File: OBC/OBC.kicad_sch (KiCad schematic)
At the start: 2 parts, among them J1 Conn_02x20_Odd_Even, U1 MPU9250

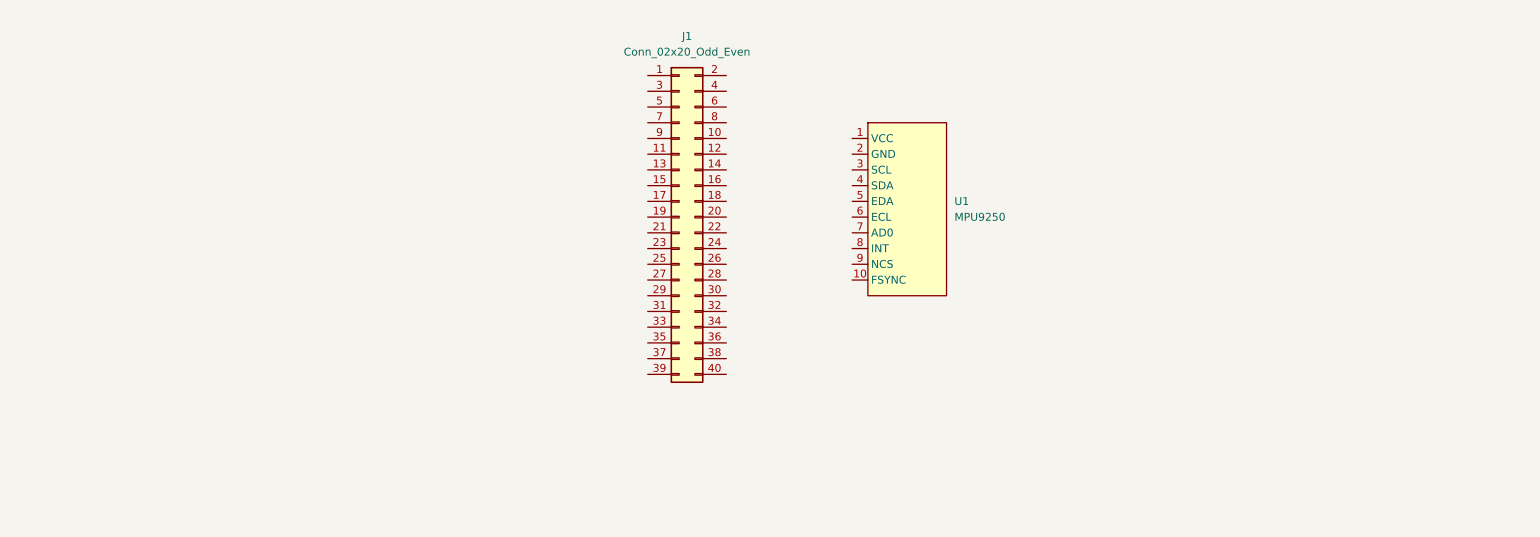
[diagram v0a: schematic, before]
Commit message: Agrega símbolo de rpi pi zero 2w
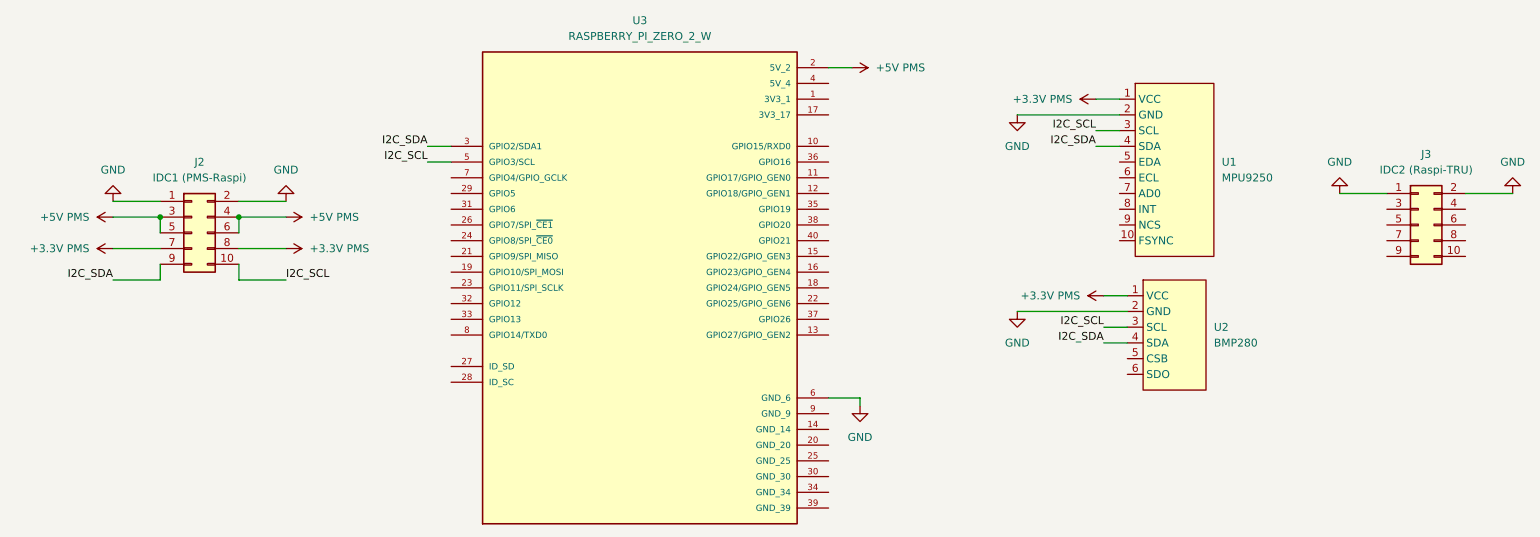
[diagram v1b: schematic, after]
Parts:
- removed J1: Conn_02x20_Odd_Even, symbol Connector_Generic:Conn_02x20_Odd_Even
- added J2: IDC1 (PMS-Raspi), symbol Connector_Generic:Conn_02x05_Odd_Even
- added J3: IDC2 (Raspi-TRU), symbol Connector_Generic:Conn_02x05_Odd_Even
- added U2: BMP280, symbol Cubesat:BMP280
- added U3: RASPBERRY_PI_ZERO_2_W, RASPBERRY_PI_ZERO_2_W:MODULE_RASPBERRY_PI_ZERO_2_W, symbol RASPBERRY_PI_ZERO_2_W:RASPBERRY_PI_ZERO_2_W
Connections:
- net +3.3V PMS: now reaches U1.1 (VCC)
- net +3.3V PMS: now also J2.7 (Pin_7), J2.8 (Pin_8), U2.1 (VCC)
- net GND: now reaches U1.2 (GND)
- net GND: now also J2.1 (Pin_1), J2.2 (Pin_2), J3.1 (Pin_1), J3.2 (Pin_2), U2.2 (GND), U3.6 (GND_6)
- net I2C_SCL: now reaches U1.3 (SCL)
- net I2C_SCL: now also J2.10 (Pin_10), U2.3 (SCL), U3.5 (GPIO3/SCL)
- net I2C_SDA: now reaches U1.4 (SDA)
- net I2C_SDA: now also J2.9 (Pin_9), U2.4 (SDA), U3.3 (GPIO2/SDA1)
- new net +5V PMS: J2.3 (Pin_3), J2.4 (Pin_4), J2.5 (Pin_5), J2.6 (Pin_6), U3.2 (5V_2)
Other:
- moved on the sheet: U1
